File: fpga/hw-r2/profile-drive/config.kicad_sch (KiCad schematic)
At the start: 23 parts, among them J4 JTAG 1x6, J6 flash service 1x7, J7 PROGRAMN button header (optio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, SW1 PROGRAMN button, U1 LFE5U-12F-6TG144C, U4 W25Q128JVSIQ, X1 25MHz XO 2520 3V3

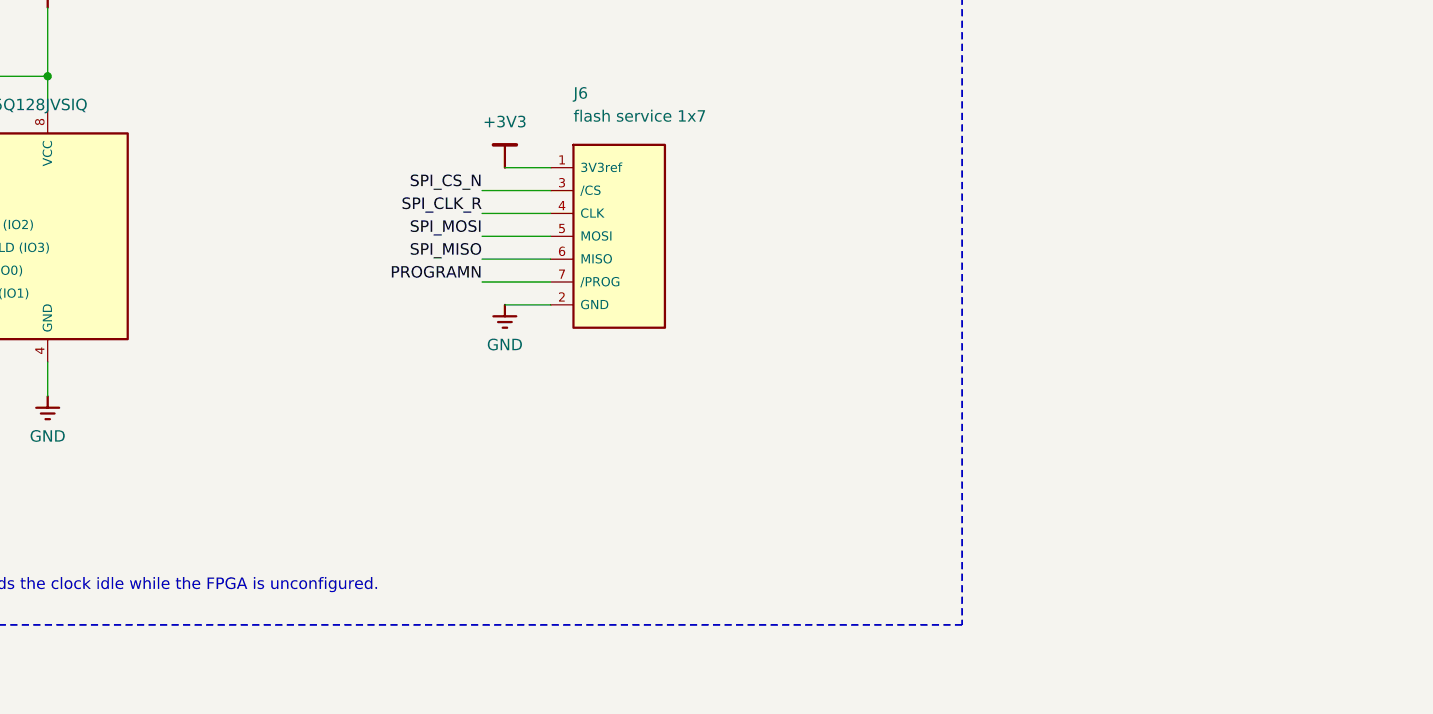
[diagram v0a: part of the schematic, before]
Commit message: fixups, tweaking
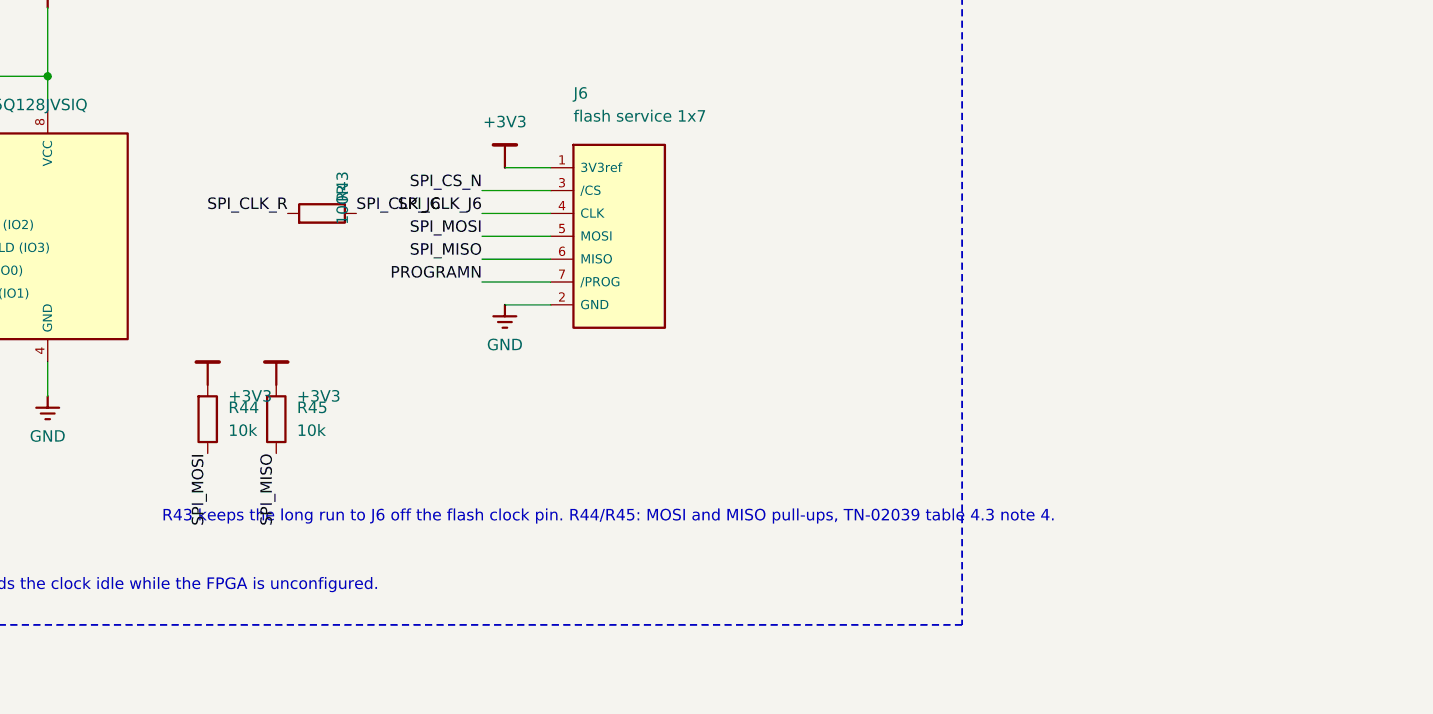
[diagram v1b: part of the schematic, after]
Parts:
- added R43: 100R, Resistor_SMD:R_0603_1608Metric, symbol device:R
- added R44, R45: 10k, Resistor_SMD:R_0603_1608Metric, symbol device:R
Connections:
- net +3V3: now also R44.1, R45.1
- net SPI_CLK_R: now also R43.1; no longer J6.4 (CLK)
- net SPI_MISO: now also R45.2
- net SPI_MOSI: now also R44.2
- new net SPI_CLK_J6: J6.4 (CLK), R43.2
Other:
- note added: "R43 keeps the long run to J6 off the flash clock pin. R44/R45: MOSI and MISO pull-ups, TN-02039 table 4.3 note 4."
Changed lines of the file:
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@@
   (label "SPI_CS_N" (at 365.76 91.44 180) (fields_autoplaced yes) (effects (font (size 1.27 1.27)) (justify right bottom)))
   (wire (pts (xy 373.38 93.98) (xy 365.76 93.98)) (stroke (width 0) (type default)))
-  (label "SPI_CLK_R" (at 365.76 93.98 180) (fields_autoplaced yes) (effects (font (size 1.27 1.27)) (justify right bottom)))
+  (label "SPI_CLK_J6" (at 365.76 93.98 180) (fields_autoplaced yes) (effects (font (size 1.27 1.27)) (justify right bottom)))
   (wire (pts (xy 373.38 96.52) (xy 365.76 96.52)) (stroke (width 0) (type default)))
   (label "SPI_MOSI" (at 365.76 96.52 180) (fields_autoplaced yes) (effects (font (size 1.27 1.27)) (justify right bottom)))
@@
   (label "CLK25" (at 321.31 180.34 0) (fields_autoplaced yes) (effects (font (size 1.27 1.27)) (justify left bottom)))
   (text "CLK25 enters PCLKT0_0 (pin 128); the design multiplies it to 50 MHz in the PLL." (exclude_from_sim no) (at 256.54 198.12 0) (effects (font (size 1.27 1.27)) (justify left top)))
+  (symbol (lib_id "device:R") (at 347.98 93.98 90) (unit 1)
+    (exclude_from_sim no) (in_bom yes) (on_board yes) (dnp no)
+    (property "Reference" "R43" (at 350.27 92.71 0) (effects (font (size 1.27 1.27)) (justify left)))
+    (property "Value" "100R" (at 350.27 95.25 0) (effects (font (size 1.27 1.27)) (justify left)))
+    (property "Footprint" "Resistor_SMD:R_0603_1608Metric" (at 347.98 93.98 0) (effects (font (size 1.27 1.27)) hide))
+    (property "Datasheet" "" (at 347.98 93.98 0) (effects (font (size 1.27 1.27)) hide))
+    (property "Description" "resistor" (at 347.98 93.98 0) (effects (font (size 1.27 1.27)) hide))
+    (pin "1")
+    (pin "2")
+    (instances (project "profile-drive" (path "/a55e218f-75e5-4ac7-a1a1-30827bd7ace5/695229fb-70b3-528e-9b1e-e2ca33d5906b" (reference "R43") (unit 1))))
+  )
+  (label "SPI_CLK_R" (at 344.17 93.98 180) (fields_autoplaced yes) (effects (font (size 1.27 1.27)) (justify right bottom)))
+  (label "SPI_CLK_J6" (at 351.79 93.98 0) (fields_autoplaced yes) (effects (font (size 1.27 1.27)) (justify left bottom)))
+  (symbol (lib_id "device:R") (at 335.28 116.84 0) (unit 1)
+    (exclude_from_sim no) (in_bom yes) (on_board yes) (dnp no)
+    (property "Reference" "R44" (at 337.57 115.57 0) (effects (font (size 1.27 1.27)) (justify left)))
+    (property "Value" "10k" (at 337.57 118.11 0) (effects (font (size 1.27 1.27)) (justify left)))
+    (property "Footprint" "Resistor_SMD:R_0603_1608Metric" (at 335.28 116.84 0) (effects (font (size 1.27 1.27)) hide))
+    (property "Datasheet" "" (at 335.28 116.84 0) (effects (font (size 1.27 1.27)) hide))
+    (property "Description" "resistor" (at 335.28 116.84 0) (effects (font (size 1.27 1.27)) hide))
+    (pin "1")
+    (pin "2")
+    (instances (project "profile-drive" (path "/a55e218f-75e5-4ac7-a1a1-30827bd7ace5/695229fb-70b3-528e-9b1e-e2ca33d5906b" (reference "R44") (unit 1))))
+  )
+  (symbol (lib_id "device:P3V3") (at 335.28 113.03 0) (unit 1)
+    (exclude_from_sim no) (in_bom no) (on_board yes) (dnp no)
+    (property "Reference" "#PWR905" (at 337.57 111.76 0) (effects (font (size 1.27 1.27)) hide))
+    (property "Value" "+3V3" (at 337.57 114.3 0) (effects (font (size 1.27 1.27)) (justify left)))
+    (property "Footprint" "" (at 335.28 113.03 0) (effects (font (size 1.27 1.27)) hide))
+    (property "Datasheet" "" (at 335.28 113.03 0) (effects (font (size 1.27 1.27)) hide))
+    (property "Description" "" (at 335.28 113.03 0) (effects (font (size 1.27 1.27)) hide))
+    (pin "1")
+    (instances (project "profile-drive" (path "/a55e218f-75e5-4ac7-a1a1-30827bd7ace5/695229fb-70b3-528e-9b1e-e2ca33d5906b" (reference "#PWR905") (unit 1))))
+  )
+  (label "SPI_MOSI" (at 335.28 120.65 270) (fields_autoplaced yes) (effects (font (size 1.27 1.27)) (justify right bottom)))
+  (symbol (lib_id "device:R") (at 342.9 116.84 0) (unit 1)
+    (exclude_from_sim no) (in_bom yes) (on_board yes) (dnp no)
+    (property "Reference" "R45" (at 345.19 115.57 0) (effects (font (size 1.27 1.27)) (justify left)))
+    (property "Value" "10k" (at 345.19 118.11 0) (effects (font (size 1.27 1.27)) (justify left)))
+    (property "Footprint" "Resistor_SMD:R_0603_1608Metric" (at 342.9 116.84 0) (effects (font (size 1.27 1.27)) hide))
+    (property "Datasheet" "" (at 342.9 116.84 0) (effects (font (size 1.27 1.27)) hide))
+    (property "Description" "resistor" (at 342.9 116.84 0) (effects (font (size 1.27 1.27)) hide))
+    (pin "1")
+    (pin "2")
+    (instances (project "profile-drive" (path "/a55e218f-75e5-4ac7-a1a1-30827bd7ace5/695229fb-70b3-528e-9b1e-e2ca33d5906b" (reference "R45") (unit 1))))
+  )
+  (symbol (lib_id "device:P3V3") (at 342.9 113.03 0) (unit 1)
+    (exclude_from_sim no) (in_bom no) (on_board yes) (dnp no)
+    (property "Reference" "#PWR906" (at 345.19 111.76 0) (effects (font (size 1.27 1.27)) hide))
+    (property "Value" "+3V3" (at 345.19 114.3 0) (effects (font (size 1.27 1.27)) (justify left)))
+    (property "Footprint" "" (at 342.9 113.03 0) (effects (font (size 1.27 1.27)) hide))
+    (property "Datasheet" "" (at 342.9 113.03 0) (effects (font (size 1.27 1.27)) hide))
+    (property "Description" "" (at 342.9 113.03 0) (effects (font (size 1.27 1.27)) hide))
+    (pin "1")
+    (instances (project "profile-drive" (path "/a55e218f-75e5-4ac7-a1a1-30827bd7ace5/695229fb-70b3-528e-9b1e-e2ca33d5906b" (reference "#PWR906") (unit 1))))
+  )
+  (label "SPI_MISO" (at 342.9 120.65 270) (fields_autoplaced yes) (effects (font (size 1.27 1.27)) (justify right bottom)))
+  (text "R43 keeps the long run to J6 off the flash clock pin. R44/R45: MOSI and MISO pull-ups, TN-02039 table 4.3 note 4." (exclude_from_sim no) (at 330.2 127 0) (effects (font (size 1.27 1.27)) (justify left top)))
   (sheet_instances (path "/" (page "4")))
   (symbol (lib_id "device:Header_2PIN") (at 144.78 127 0) (unit 1)
